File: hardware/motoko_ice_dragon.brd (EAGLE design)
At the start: 93 x 88 mm, 138 parts, among them Q1 8MHz, Q10 20mA/30V, Q11 20mA/30V, Q2 BSS138TOP, Q3 BSS138TOP, Q4 20mA/30V, Q5 20mA/30V, Q6 20mA/30V, Q7 20mA/30V, Q8 20mA/30V, Q9 20mA/30V, U1 MP6540HA, U2 STM32_STM32F722XX, U3 MP6540HA, U4 AP63203

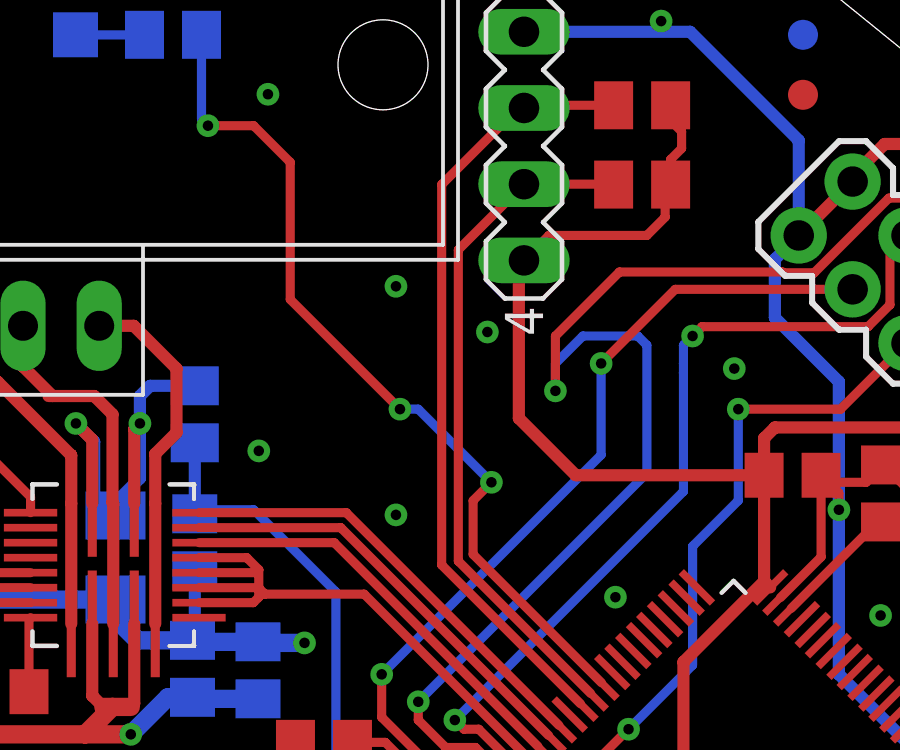
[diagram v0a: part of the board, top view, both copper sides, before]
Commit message: gyro tests
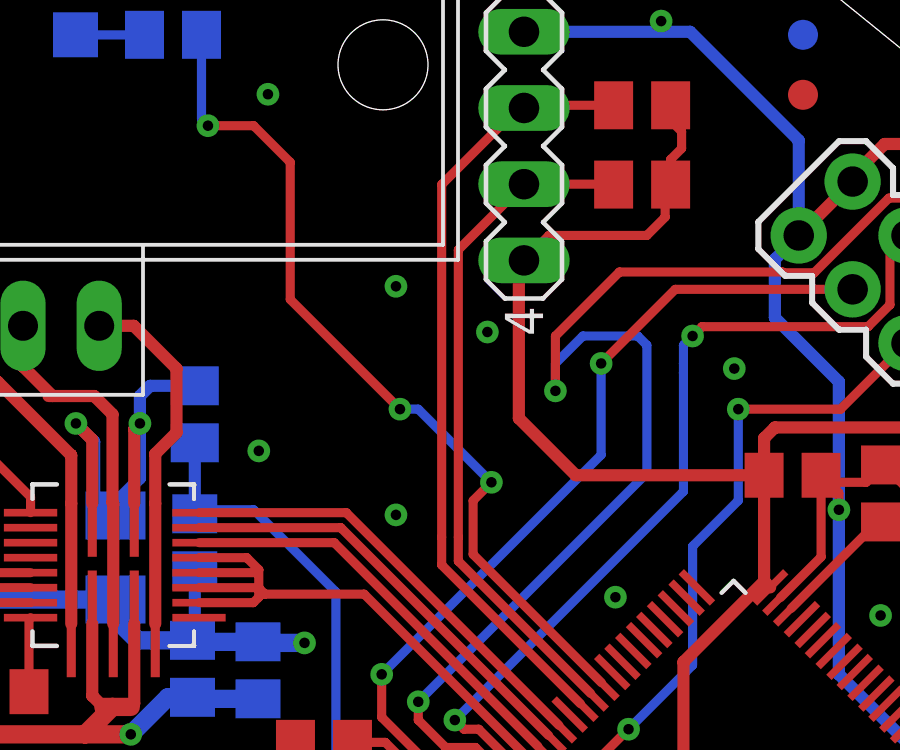
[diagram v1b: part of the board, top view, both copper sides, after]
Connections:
- net L_SCL: now also L_ENCODER.3, R37.2, U2.61; no longer L_ENCODER.2, R4.2, U2.62
- net L_SDA: now also L_ENCODER.2, R4.2, U2.62; no longer L_ENCODER.3, R37.2, U2.61
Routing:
- net L_SDA: track 22.7 -> 26.1 mm
- net L_SCL: track 26.1 -> 22.7 mm
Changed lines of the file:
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@@
 <wire x1="9.144" y1="47.8892" x2="9.718" y2="48.4632" width="0.6096" layer="16"/>
 </signal>
-<signal name="L_SDA">
-<contactref element="U2" pad="61"/>
+<signal name="L_SCL">
 <contactref element="L_ENCODER" pad="3"/>
-<wire x1="31.51065625" y1="53.456259375" x2="31.51065625" y2="63.83265625" width="0.3048" layer="1"/>
+<wire x1="31.51065625" y1="54.2544" x2="31.51065625" y2="63.83265625" width="0.3048" layer="1"/>
 <wire x1="31.51065625" y1="63.83265625" x2="33.6992" y2="66.0212" width="0.3048" layer="1"/>
 <contactref element="R37" pad="2"/>
 <wire x1="33.6992" y1="66.0212" x2="36.6736" y2="66.0212" width="0.3048" layer="1"/>
 <wire x1="36.6736" y1="66.0212" x2="36.6876" y2="66.0072" width="0.3048" layer="1"/>
+<contactref element="U2" pad="61"/>
 <wire x1="35.9246625" y1="49.042253125" x2="31.51065625" y2="53.456259375" width="0.3048" layer="1"/>
-</signal>
-<signal name="L_SCL">
-<contactref element="U2" pad="62"/>
-<wire x1="35.5834125" y1="48.701003125" x2="30.956" y2="53.328415625" width="0.3048" layer="1"/>
-<wire x1="30.956" y1="53.328415625" x2="30.956" y2="66.008" width="0.3048" layer="1"/>
-<wire x1="33.5092" y1="68.5612" x2="30.956" y2="66.008" width="0.3048" layer="1"/>
-<contactref element="L_ENCODER" pad="2"/>
-<contactref element="R4" pad="2"/>
-<wire x1="33.6992" y1="68.5612" x2="33.7892" y2="68.6512" width="0.3048" layer="1"/>
-<wire x1="33.7892" y1="68.6512" x2="36.6876" y2="68.6512" width="0.3048" layer="1"/>
-<wire x1="33.6992" y1="68.5612" x2="33.5092" y2="68.5612" width="0.3048" layer="1"/>
+<wire x1="31.51065625" y1="53.456259375" x2="31.51065625" y2="54.2544" width="0.3048" layer="1"/>
 </signal>
 <signal name="N$9">
@@
 <wire x1="31.25" y1="37.6348" x2="31.25" y2="36.9" width="0.3048" layer="1"/>
 </signal>
+<signal name="L_SDA">
+<contactref element="L_ENCODER" pad="2"/>
+<contactref element="R4" pad="2"/>
+<wire x1="30.956" y1="54.2544" x2="30.956" y2="66.008" width="0.3048" layer="1"/>
+<wire x1="33.5092" y1="68.5612" x2="30.956" y2="66.008" width="0.3048" layer="1"/>
+<wire x1="33.6992" y1="68.5612" x2="33.7892" y2="68.6512" width="0.3048" layer="1"/>
+<wire x1="33.7892" y1="68.6512" x2="36.6876" y2="68.6512" width="0.3048" layer="1"/>
+<wire x1="33.6992" y1="68.5612" x2="33.5092" y2="68.5612" width="0.3048" layer="1"/>
+<contactref element="U2" pad="62"/>
+<wire x1="35.5834125" y1="48.701003125" x2="30.956" y2="53.328415625" width="0.3048" layer="1"/>
+<wire x1="30.956" y1="53.328415625" x2="30.956" y2="54.2544" width="0.3048" layer="1"/>
+</signal>
 </signals>
